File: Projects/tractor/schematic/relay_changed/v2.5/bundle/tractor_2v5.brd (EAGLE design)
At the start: 66.5 x 45.5 mm, 80 parts, among them IC1 PIC16F1824, IC2 33063A, K2 RL3531RL3, Q1 IRLML2402, Q2 IRLML2402, Q3 IRLML2402, Q4 2N2222

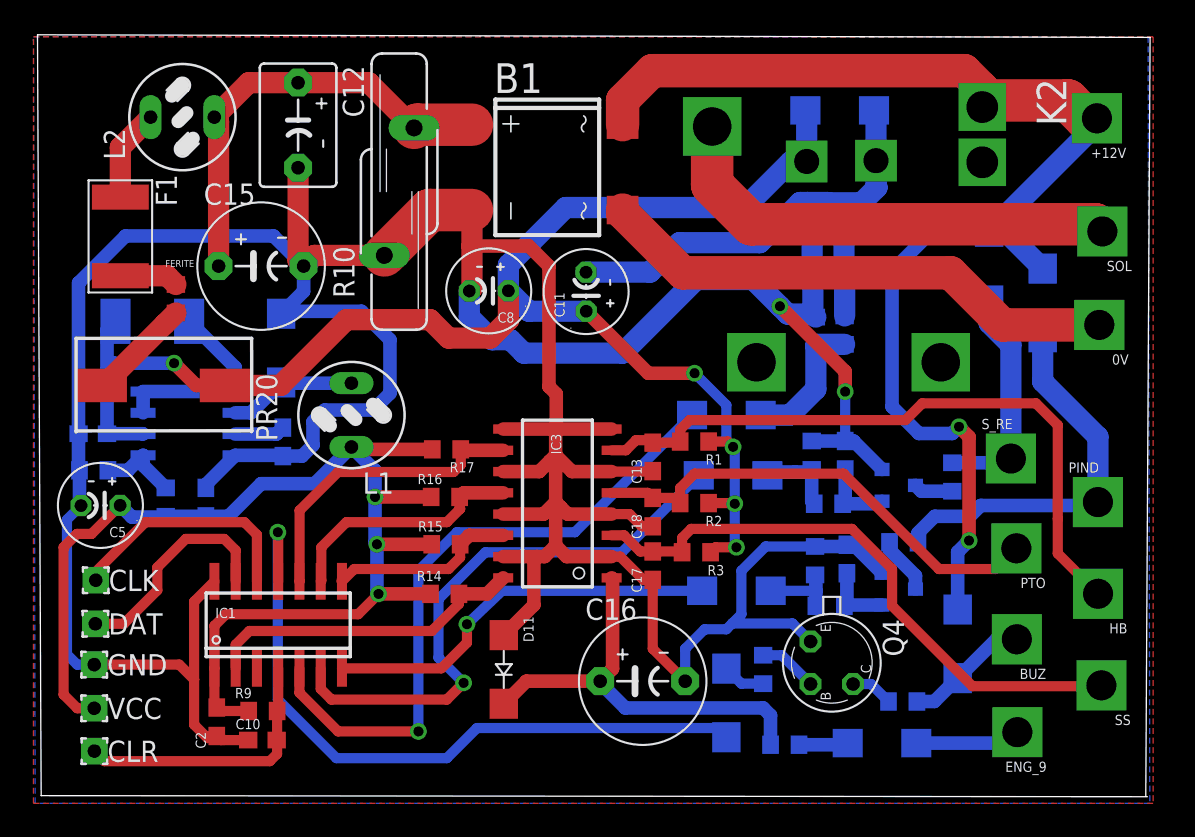
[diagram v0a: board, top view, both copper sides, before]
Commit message: Version2.5 modified schematic and code updated
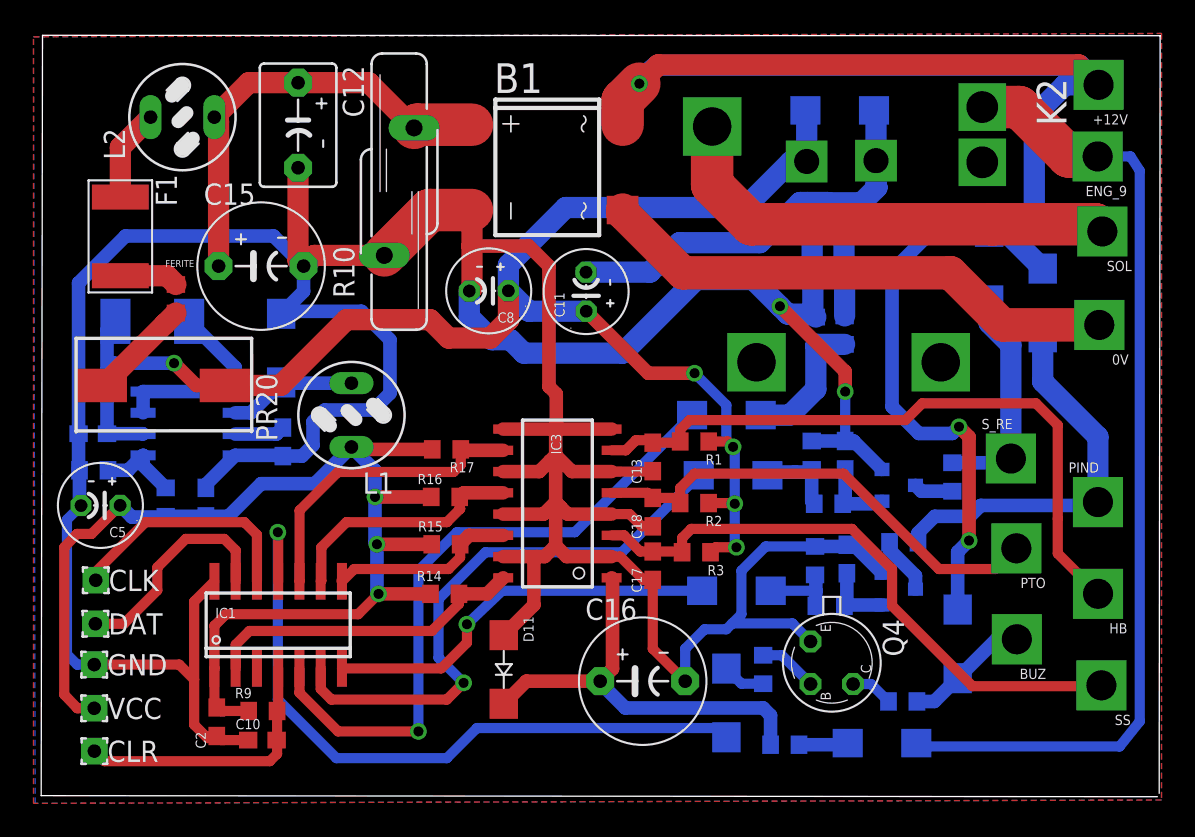
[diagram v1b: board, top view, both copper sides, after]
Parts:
- moved ENG_9 34.7 mm to (63.7, 38.4)
- moved +12V 2.00 mm to (63.7, 42.6)
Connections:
- removed net N$35: D12.A, ENG_9.1
- new net ENG_12V: D12.A, ENG_9.1, K2.NC
- net 12V_8: no longer K2.NC
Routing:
- net ENG_12V: track 0.00 -> 58.1 mm
- net 12V_8: track 77.7 -> 109.0 mm, vias 2 -> 3
- net N$35: track 6.31 -> 0.00 mm
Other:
- board size 66.5 x 45.5 mm -> 66.9 x 45.5 mm
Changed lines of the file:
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@@
 <setting verticaltext="up"/>
 </settings>
-<grid distance="0.1" unitdist="mm" unit="mm" style="lines" multiple="1" display="no" altdistance="0.025" altunitdist="inch" altunit="mm"/>
+<grid distance="0.01" unitdist="mm" unit="mm" style="lines" multiple="1" display="no" altdistance="0.025" altunitdist="inch" altunit="mm"/>
 <layers>
 <layer number="1" name="Top" color="4" fill="1" visible="yes" active="yes"/>
@@
 <board>
 <plain>
-<wire x1="66.817259375" y1="45.465509375" x2="0.34" y2="45.62" width="0" layer="20"/>
-<wire x1="0.34" y1="45.62" x2="0.56" y2="0.16" width="0" layer="20"/>
-<wire x1="66.56" y1="0.16" x2="66.817259375" y2="45.465509375" width="0" layer="20"/>
+<wire x1="67.417259375" y1="45.565509375" x2="0.64" y2="45.59" width="0" layer="20"/>
+<wire x1="0.64" y1="45.59" x2="0.56" y2="0.16" width="0" layer="20"/>
+<wire x1="67.36" y1="0.3" x2="67.417259375" y2="45.565509375" width="0" layer="20"/>
 <dimension x1="66.56" y1="0.16" x2="0.56" y2="0.16" x3="33.56" y3="-4.84" textsize="1.778" layer="47"/>
 <dimension x1="0.56" y1="0.16" x2="0.56" y2="45.27" x3="-9.76" y3="22.715" textsize="1.778" layer="47"/>
-<wire x1="66.657259375" y1="0.095509375" x2="0.56" y2="0.16" width="0" layer="20"/>
-<dimension x1="0.1" y1="45.5" x2="66.7" y2="45.5" x3="33.4" y3="49.5" textsize="1.778" layer="51"/>
+<wire x1="67.257259375" y1="0.095509375" x2="0.56" y2="0.16" width="0" layer="20"/>
+<dimension x1="0.64" y1="45.59" x2="67.417259375" y2="45.565509375" x3="34.029509375" y3="47.97095625" textsize="1.778" layer="51"/>
+<dimension x1="0.64" y1="45.59" x2="0.56" y2="0.16" x3="-2.659921875" y3="22.8807375" textsize="1.778" layer="51"/>
 </plain>
 <attributes>
@@
 <attribute name="VALUE" x="63.782303125" y="27.28559375" size="0.0254" layer="27" rot="R180"/>
 </element>
-<element name="+12V" library="wirepad" package="2,54/1,1" value="+12V" x="63.6407" y="40.63065625" rot="R180">
-<attribute name="VALUE" x="63.6407" y="39.63065625" size="0.0254" layer="27" rot="R180"/>
+<element name="+12V" library="wirepad" package="2,54/1,1" value="+12V" x="63.7407" y="42.63065625" rot="R180">
+<attribute name="VALUE" x="63.7407" y="41.63065625" size="0.0254" layer="27" rot="R180"/>
 </element>
 <element name="SOL" library="wirepad" package="2,54/1,1" value="" x="63.965525" y="33.872403125" rot="R180">
 <attribute name="VALUE" x="63.965525" y="32.872403125" size="0.0254" layer="27" rot="R180"/>
 </element>
-<element name="ENG_9" library="wirepad" package="2,54/1,1" value="" x="58.88544375" y="3.9530375" rot="R180">
-<attribute name="VALUE" x="58.88544375" y="2.9530375" size="0.0254" layer="27" rot="R180"/>
+<element name="ENG_9" library="wirepad" package="2,54/1,1" value="" x="63.68544375" y="38.3530375" rot="R180">
+<attribute name="VALUE" x="63.68544375" y="37.3530375" size="0.0254" layer="27" rot="R180"/>
 </element>
 <element name="PTO" library="wirepad" package="2,54/1,1" value="" x="58.826125" y="14.9380625" rot="R180">
@@
 <contactref element="R10" pad="1"/>
 <contactref element="C12" pad="2"/>
-<polygon width="0.508" layer="1" spacing="1.9304" pour="cutout" isolate="0.6096" thermals="no">
+<polygon width="0.508" layer="1" spacing="1.9304" isolate="0.6096" thermals="no">
 <vertex x="0.1" y="45.5"/>
-<vertex x="67" y="45.5"/>
-<vertex x="67" y="-0.3"/>
+<vertex x="67.5" y="45.7"/>
+<vertex x="67.5" y="-0.1"/>
 <vertex x="0.1" y="-0.3"/>
 </polygon>
-<polygon width="0.508" layer="16" spacing="1.9304" pour="cutout" isolate="0.6096">
+<polygon width="0.508" layer="16" spacing="1.9304" isolate="0.6096">
 <vertex x="0.1" y="45.5"/>
-<vertex x="66.7" y="45.5"/>
-<vertex x="66.8" y="-0.3"/>
+<vertex x="67.5" y="45.7"/>
+<vertex x="67.5" y="-0.1"/>
 <vertex x="0.2" y="-0.3"/>
 </polygon>
@@
 <wire x1="5.27594375" y1="17.50610625" x2="3.5698375" y2="15.8" width="0.6096" layer="1"/>
 <wire x1="3.5698375" y1="15.8" x2="2.7" y2="15.8" width="0.6096" layer="1"/>
-<wire x1="2.7" y1="15.8" x2="1.9" y2="15" width="0.6096" layer="1"/>
+<wire x1="2.7" y1="15.8" x2="1.94" y2="15" width="0.6096" layer="1"/>
 <wire x1="2.72" y1="5.38" x2="3.73" y2="5.38" width="0.6096" layer="1"/>
-<wire x1="1.9" y1="6.2" x2="2.72" y2="5.38" width="0.6096" layer="1"/>
-<wire x1="1.9" y1="15" x2="1.9" y2="6.2" width="0.6096" layer="1"/>
+<wire x1="1.94" y1="6.2" x2="2.72" y2="5.38" width="0.6096" layer="1"/>
+<wire x1="1.94" y1="15" x2="1.94" y2="6.2" width="0.6096" layer="1"/>
 </signal>
 <signal name="VDD">
@@
 <wire x1="63.537928125" y1="34.3" x2="63.965525" y2="33.872403125" width="2.54" layer="1"/>
 <wire x1="40.6499875" y1="36.6500125" x2="43" y2="34.3" width="2.54" layer="1"/>
-<wire x1="43" y1="34.3" x2="63.537928125" y2="34.3" width="2.54" layer="1"/>
+<wire x1="43" y1="34.3" x2="57.4" y2="34.3" width="2.54" layer="1"/>
+<wire x1="57.4" y1="34.3" x2="63.537928125" y2="34.3" width="2.54" layer="1"/>
 </signal>
 <signal name="12V_8">
@@
 <wire x1="60.4" y1="31.65" x2="58.2" y2="33.85" width="1.27" layer="16"/>
 <wire x1="58.2" y1="33.85" x2="57.2" y2="33.85" width="1.27" layer="16"/>
-<wire x1="63.6407" y1="40.2907" x2="57.2" y2="33.85" width="1.27" layer="16"/>
 <contactref element="D4" pad="K"/>
 <wire x1="57.2" y1="33.85" x2="53.75" y2="33.85" width="0.8128" layer="16"/>
@@
 <wire x1="55.32" y1="14.72" x2="56" y2="15.4" width="0.8128" layer="16"/>
 <wire x1="35.1" y1="40.45" x2="35.3" y2="40.25" width="1.27" layer="1"/>
-<contactref element="K2" pad="NC"/>
-<wire x1="63.6407" y1="40.63065625" x2="63.6407" y2="40.2907" width="1.27" layer="16"/>
-<wire x1="63.6407" y1="40.63065625" x2="62.96934375" y2="40.63065625" width="2.54" layer="1"/>
-<wire x1="62.96934375" y1="40.63065625" x2="61.9" y2="41.7" width="2.54" layer="1"/>
-<wire x1="61.9" y1="41.7" x2="57.187309375" y2="41.7" width="2.54" layer="1"/>
-<wire x1="57.187309375" y1="41.7" x2="56.7899875" y2="41.302678125" width="2.54" layer="1"/>
-<wire x1="56.7899875" y1="41.302678125" x2="56.7899875" y2="42.4100125" width="2" layer="1"/>
-<wire x1="56.7899875" y1="42.4100125" x2="55.724715625" y2="43.475284375" width="2" layer="1"/>
-<wire x1="55.724715625" y1="43.475284375" x2="37.075284375" y2="43.475284375" width="2" layer="1"/>
-<wire x1="35.3" y1="41.7" x2="35.3" y2="40.25" width="2" layer="1"/>
-<wire x1="37.075284375" y1="43.475284375" x2="35.3" y2="41.7" width="2" layer="1"/>
+<wire x1="63.7407" y1="42.63065625" x2="61.73065625" y2="42.63065625" width="1.27" layer="16"/>
+<wire x1="59.9" y1="40.8" x2="59.9" y2="34.8" width="1.27" layer="16"/>
+<wire x1="59.9" y1="34.8" x2="58.95" y2="33.85" width="1.27" layer="16"/>
+<wire x1="58.95" y1="33.85" x2="57.2" y2="33.85" width="1.27" layer="16"/>
+<wire x1="61.73065625" y1="42.63065625" x2="59.9" y2="40.8" width="1.27" layer="16"/>
+<wire x1="62.546928125" y1="43.824428125" x2="63.7407" y2="42.63065625" width="1.27" layer="1"/>
+<wire x1="62.6" y1="43.8" x2="37.4" y2="43.8" width="1.27" layer="16"/>
+<wire x1="62.6" y1="43.8" x2="63.8" y2="42.6" width="1.27" layer="16"/>
+<wire x1="35.3" y1="40.25" x2="35.3" y2="41.7" width="2.54" layer="1"/>
+<wire x1="35.3" y1="41.7" x2="36.3" y2="42.7" width="2.54" layer="1"/>
+<wire x1="37.4" y1="43.8" x2="36.3" y2="42.9" width="1.27" layer="16"/>
+<wire x1="36.3" y1="42.9" x2="36.3" y2="42.7" width="1.27" layer="16"/>
+<via x="36.3" y="42.7" extent="1-16" drill="0.6" diameter="1"/>
+<wire x1="36.3" y1="42.7" x2="37.424428125" y2="43.824428125" width="1.27" layer="1"/>
+<wire x1="37.424428125" y1="43.824428125" x2="62.546928125" y2="43.824428125" width="1.27" layer="1"/>
 </signal>
 <signal name="N$3">
@@
 <wire x1="58.25" y1="20.05" x2="58.5" y2="20.3" width="0.8128" layer="16"/>
 </signal>
-<signal name="N$35">
+<signal name="ENG_12V">
 <contactref element="ENG_9" pad="1"/>
 <contactref element="D12" pad="A"/>
-<wire x1="52.85" y1="3.3" x2="58.23240625" y2="3.3" width="0.8128" layer="16"/>
-<wire x1="58.23240625" y1="3.3" x2="58.88544375" y2="3.9530375" width="0.8128" layer="16"/>
+<contactref element="K2" pad="NC"/>
+<wire x1="56.7899875" y1="41.302678125" x2="58.997321875" y2="41.302678125" width="2.54" layer="1"/>
+<wire x1="61.9469625" y1="38.3530375" x2="63.68544375" y2="38.3530375" width="2.54" layer="1"/>
+<wire x1="58.997321875" y1="41.302678125" x2="61.9469625" y2="38.3530375" width="2.54" layer="1"/>
+<wire x1="63.68544375" y1="38.3530375" x2="65.6469625" y2="38.3530375" width="0.6096" layer="16"/>
+<wire x1="65.6469625" y1="38.3530375" x2="66.2" y2="37.5" width="0.6096" layer="16"/>
+<wire x1="66.2" y1="37.5" x2="66.2" y2="4.6" width="0.6096" layer="16"/>
+<wire x1="66.2" y1="4.6" x2="65" y2="3.1" width="0.6096" layer="16"/>
+<wire x1="65" y1="3.1" x2="53.05" y2="3.1" width="0.6096" layer="16"/>
+<wire x1="53.05" y1="3.1" x2="52.85" y2="3.3" width="0.6096" layer="16"/>
 </signal>
 <signal name="N$36">
